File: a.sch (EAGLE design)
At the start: 30 parts, among them CON1 PINHEAD_1X04-2.54, CON2 PINHEAD_1X08-2.54, SW1 TACT_SWITCH-1-1825910-4, SW2 TACT_SWITCH-1-1825910-4, X3 PINHEAD_1X06-2-MALE, X4 PINHEAD_2X03-PTH-2.54

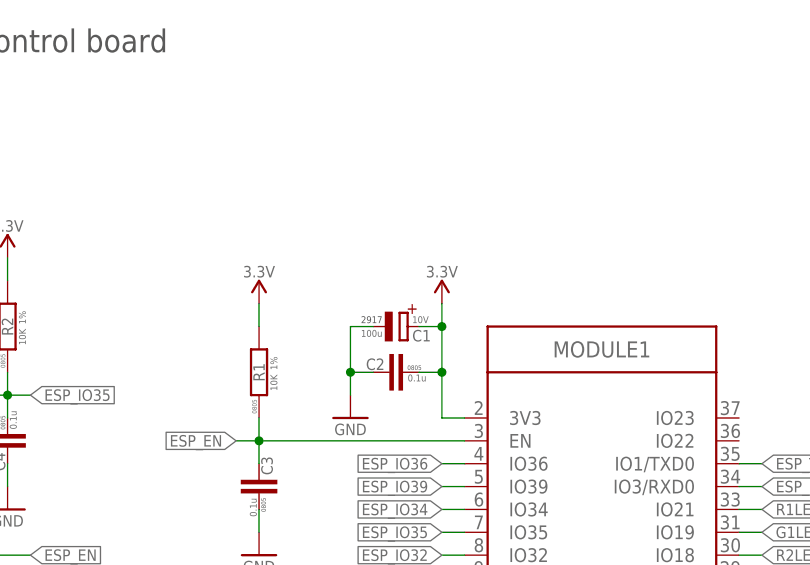
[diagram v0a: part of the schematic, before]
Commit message: preRelease minor fixes
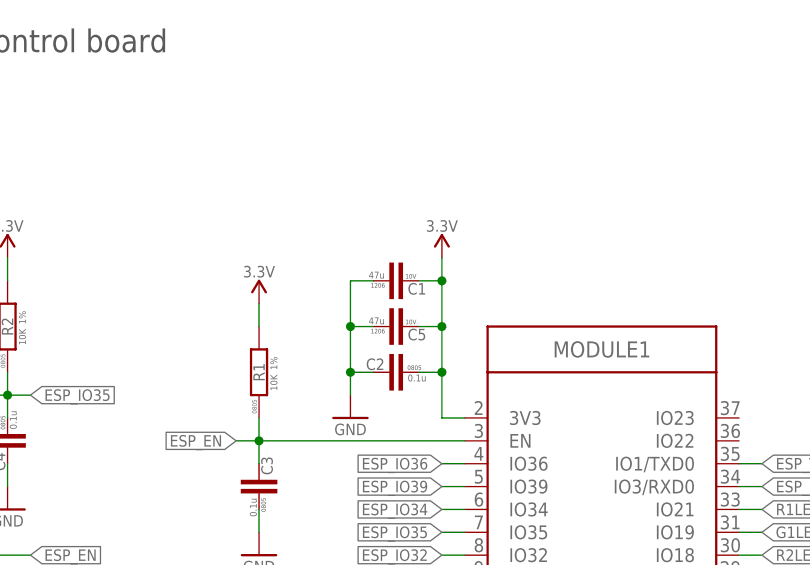
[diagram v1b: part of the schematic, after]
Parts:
- added C5: 47u, rc:C-1206
- C1: value 100u -> 47u; device rc:CPOL-2917 -> rc:C-1206
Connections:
- net GND: now also C1.1, C5.1; no longer C1.-
- net VDD_3V3: now also C1.2, C5.2; no longer C1.+
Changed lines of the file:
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@@
 <part name="C2" library="rc" library_urn="urn:adsk.eagle:library:2539423" deviceset="C" device="-0805" package3d_urn="urn:adsk.eagle:package:2539460/3" value="0.1u"/>
 <part name="GND3" library="supply_symbols" library_urn="urn:adsk.eagle:library:5017758" deviceset="GND" device="" value="GND"/>
-<part name="C1" library="rc" library_urn="urn:adsk.eagle:library:2539423" deviceset="CPOL" device="-2917" package3d_urn="urn:adsk.eagle:package:2539466/2" value="100u">
-<attribute name="VOLTAGE" value="10V"/>
-</part>
 <part name="CON1" library="pinhead" library_urn="urn:adsk.eagle:library:2540341" deviceset="PINHEAD_1X04" device="-2.54" package3d_urn="urn:adsk.eagle:package:2540383/2"/>
 <part name="CON2" library="pinhead" library_urn="urn:adsk.eagle:library:2540341" deviceset="PINHEAD_1X08" device="-2.54" package3d_urn="urn:adsk.eagle:package:2540379/4"/>
@@
 <part name="R15" library="rc" library_urn="urn:adsk.eagle:library:2539423" deviceset="R" device="-0805" package3d_urn="urn:adsk.eagle:package:2539455/2" technology="-1%" value="1K"/>
 <part name="+P8" library="supply_symbols" library_urn="urn:adsk.eagle:library:5017758" deviceset="3.3V" device=""/>
+<part name="C5" library="rc" library_urn="urn:adsk.eagle:library:2539423" deviceset="C" device="-1206" package3d_urn="urn:adsk.eagle:package:2539459/2" value="47u">
+<attribute name="VOLTAGE" value="10V"/>
+</part>
+<part name="C1" library="rc" library_urn="urn:adsk.eagle:library:2539423" deviceset="C" device="-1206" package3d_urn="urn:adsk.eagle:package:2539459/2" value="47u">
+<attribute name="VOLTAGE" value="10V"/>
+</part>
 </parts>
 <sheets>
@@
 <attribute name="MANF#" x="119.38" y="92.71" size="1.27" layer="95" font="vector" align="center"/>
 </instance>
-<instance part="+P1" gate="G$1" x="101.6" y="142.24" smashed="yes">
-<attribute name="VALUE" x="101.6" y="145.796" size="1.27" layer="96" font="vector" ratio="15" align="center"/>
+<instance part="+P1" gate="G$1" x="101.6" y="147.32" smashed="yes">
+<attribute name="VALUE" x="101.6" y="150.876" size="1.27" layer="96" font="vector" ratio="15" align="center"/>
 </instance>
 <instance part="GND1" gate="1" x="137.16" y="91.44" smashed="yes">
@@
 <attribute name="VALUE" x="91.44" y="128.27" size="1.27" layer="96" font="vector" ratio="15" align="center"/>
 </instance>
-<instance part="C1" gate="G$1" x="96.52" y="139.7" smashed="yes">
-<attribute name="NAME" x="98.298" y="138.684" size="1.27" layer="95" font="vector" align="center-left"/>
-<attribute name="VALUE" x="94.996" y="138.938" size="0.762" layer="96" font="vector" rot="R180" align="center-left"/>
-<attribute name="PACKAGE" x="94.996" y="140.462" size="0.762" layer="97" font="vector" align="center-right"/>
-<attribute name="VOLTAGE" x="98.298" y="140.462" size="0.762" layer="96" font="vector" align="center-left"/>
-</instance>
 <instance part="CON1" gate="G$1" x="58.42" y="43.18" smashed="yes" rot="MR180">
 <attribute name="NAME" x="60.96" y="29.21" size="1.778" layer="95" font="vector" ratio="15" rot="MR180" align="center"/>
@@
 <attribute name="VALUE" x="236.22" y="97.536" size="1.27" layer="96" font="vector" ratio="15" rot="MR0" align="center"/>
 </instance>
+<instance part="C5" gate="G$1" x="96.52" y="139.7" smashed="yes">
+<attribute name="NAME" x="97.79" y="138.811" size="1.27" layer="95" font="vector" align="center-left"/>
+<attribute name="VALUE" x="95.25" y="139.954" size="0.762" layer="96" font="vector" align="bottom-right"/>
+<attribute name="PACKAGE" x="94.488" y="139.192" size="0.508" layer="97" font="vector" rot="R180" align="center"/>
+<attribute name="VOLTAGE" x="97.536" y="140.208" size="0.508" layer="97" font="vector" align="center-left"/>
+<attribute name="ALLOCATED" x="96.52" y="142.24" size="0.508" layer="97" font="vector" align="center"/>
+</instance>
+<instance part="C1" gate="G$1" x="96.52" y="144.78" smashed="yes">
+<attribute name="NAME" x="97.79" y="143.891" size="1.27" layer="95" font="vector" align="center-left"/>
+<attribute name="VALUE" x="95.25" y="145.034" size="0.762" layer="96" font="vector" align="bottom-right"/>
+<attribute name="PACKAGE" x="94.488" y="144.272" size="0.508" layer="97" font="vector" rot="R180" align="center"/>
+<attribute name="VOLTAGE" x="97.536" y="145.288" size="0.508" layer="97" font="vector" align="center-left"/>
+<attribute name="ALLOCATED" x="96.52" y="147.32" size="0.508" layer="97" font="vector" align="center"/>
+</instance>
 </instances>
 <busses>
@@
 </segment>
 <segment>
-<pinref part="C1" gate="G$1" pin="-"/>
 <wire x1="93.98" y1="139.7" x2="91.44" y2="139.7" width="0.1524" layer="91"/>
 <pinref part="C2" gate="G$1" pin="2"/>
@@
 <wire x1="91.44" y1="139.7" x2="91.44" y2="134.62" width="0.1524" layer="91"/>
 <junction x="91.44" y="134.62"/>
+<pinref part="C5" gate="G$1" pin="1"/>
+<pinref part="C1" gate="G$1" pin="1"/>
+<wire x1="93.98" y1="144.78" x2="91.44" y2="144.78" width="0.1524" layer="91"/>
+<wire x1="91.44" y1="144.78" x2="91.44" y2="139.7" width="0.1524" layer="91"/>
+<junction x="91.44" y="139.7"/>
 </segment>
 <segment>
@@
 <wire x1="101.6" y1="134.62" x2="101.6" y2="139.7" width="0.1524" layer="91"/>
 <pinref part="C2" gate="G$1" pin="1"/>
-<wire x1="101.6" y1="139.7" x2="101.6" y2="142.24" width="0.1524" layer="91"/>
+<wire x1="101.6" y1="139.7" x2="101.6" y2="144.78" width="0.1524" layer="91"/>
+<wire x1="101.6" y1="144.78" x2="101.6" y2="147.32" width="0.1524" layer="91"/>
 <wire x1="99.06" y1="134.62" x2="101.6" y2="134.62" width="0.1524" layer="91"/>
 <junction x="101.6" y="134.62"/>
-<pinref part="C1" gate="G$1" pin="+"/>
 <wire x1="99.06" y1="139.7" x2="101.6" y2="139.7" width="0.1524" layer="91"/>
 <junction x="101.6" y="139.7"/>
 <wire x1="101.6" y1="134.62" x2="101.6" y2="129.54" width="0.1524" layer="91"/>
 <wire x1="101.6" y1="129.54" x2="104.14" y2="129.54" width="0.1524" layer="91"/>
-</segment>
-<segment>
+<pinref part="C5" gate="G$1" pin="2"/>
+<pinref part="C1" gate="G$1" pin="2"/>
+<wire x1="99.06" y1="144.78" x2="101.6" y2="144.78" width="0.1524" layer="91"/>
+<junction x="101.6" y="144.78"/>
+</segment>
+<segment>
